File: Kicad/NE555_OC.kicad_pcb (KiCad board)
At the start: 2 copper layers, 22.9 x 20.7 mm, 16 parts, among them J1 Conn_01x02_Male, J2 Conn_01x02_Male, Q1 MMBT3904, U1 NE555D, U2 AP1117-5

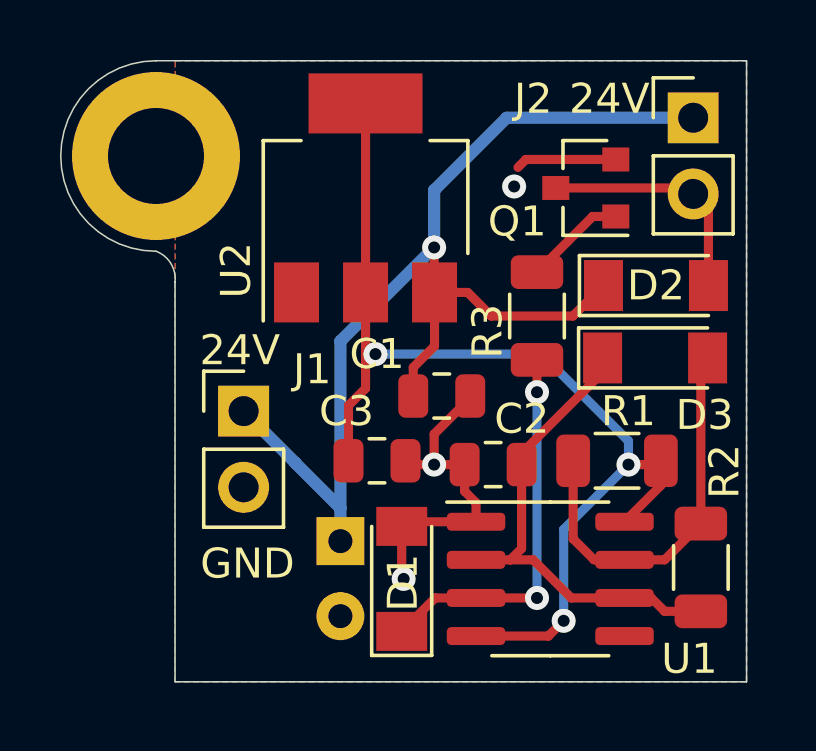
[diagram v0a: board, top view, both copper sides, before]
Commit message: Add files via upload
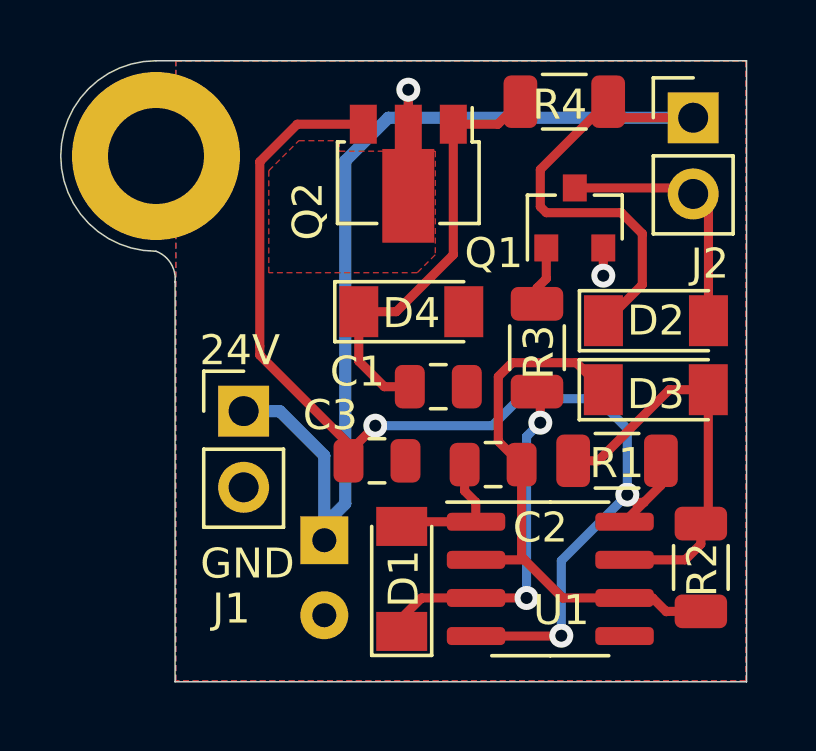
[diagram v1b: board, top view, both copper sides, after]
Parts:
- removed U2: AP1117-5, Package_TO_SOT_SMD:SOT-223-3_TabPin2
- added D4: 5V6, Diode_SMD:D_MiniMELF, F.Cu at (55.5, 85.2)
- added G***: LOGO, libs:KBS, B.Cu at (58.4, 86.1)
- added Q2: BCX56, Package_TO_SOT_SMD:SOT-89-3, F.Cu at (55.4, 80.6)
- added R4: 8k2, Resistor_SMD:R_1206_3216Metric, F.Cu at (60.6, 78.2)
- moved D2 1.17 mm to (63.7, 85.5)
- moved Q1 1.13 mm to (61.0, 82.1), turned to 90 degrees
- moved D3 1.06 mm to (63.6, 87.8)
- moved R3 1.06 mm to (59.7, 86.4)
- moved C4 0.54 mm to (52.6, 92.8)
- moved C1 0.33 mm to (56.4, 87.7)
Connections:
- C1 pad 1: +24V -> Net-(C1-Pad1)
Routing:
- net Net-(C1-Pad1): track 0.00 -> 14.5 mm
- net +24V: track 38.8 -> 48.2 mm
- net GND: track 14.6 -> 5.53 mm, vias 3 -> 1
- net +5V: track 35.9 -> 39.7 mm
- net Net-(C2-Pad1): track 16.2 -> 18.7 mm
- net Net-(Q1-Pad1): track 3.39 -> 1.99 mm
- net Net-(D1-Pad1): track 12.9 -> 12.0 mm
- net Net-(D2-Pad2): track 7.93 -> 8.47 mm
- added copper zone on F.Cu, net +24V
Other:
- board text added: "NE555 OC REL"
- board text added: "OC"
- board text removed: "NE555 OC REL KBS 2022"
